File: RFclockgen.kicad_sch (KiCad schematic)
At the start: 13 parts, among them J1 Conn_01x04_Pin, J3 Conn_01x02_Pin, U3 AP2112K-3.3, U4 ESP32-C6-WROOM-1-N8

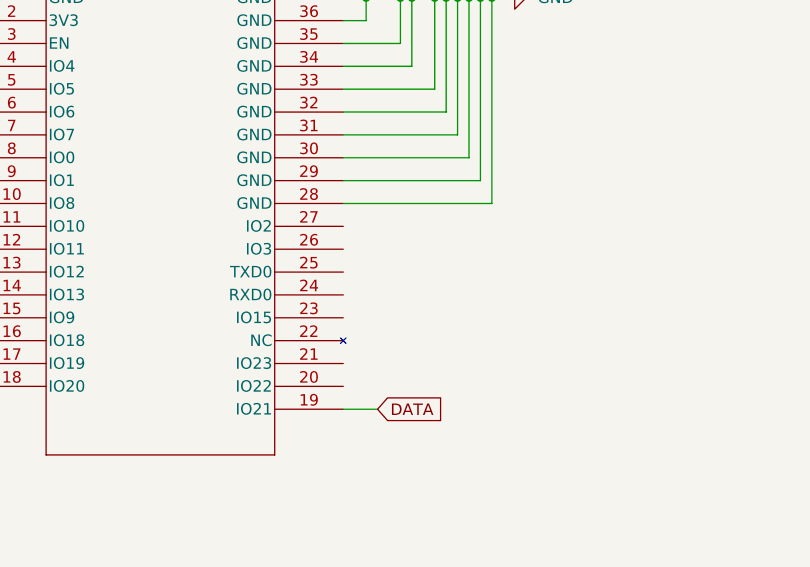
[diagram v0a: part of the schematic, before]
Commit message: Actually started on PCB layout
Started the USB C connector
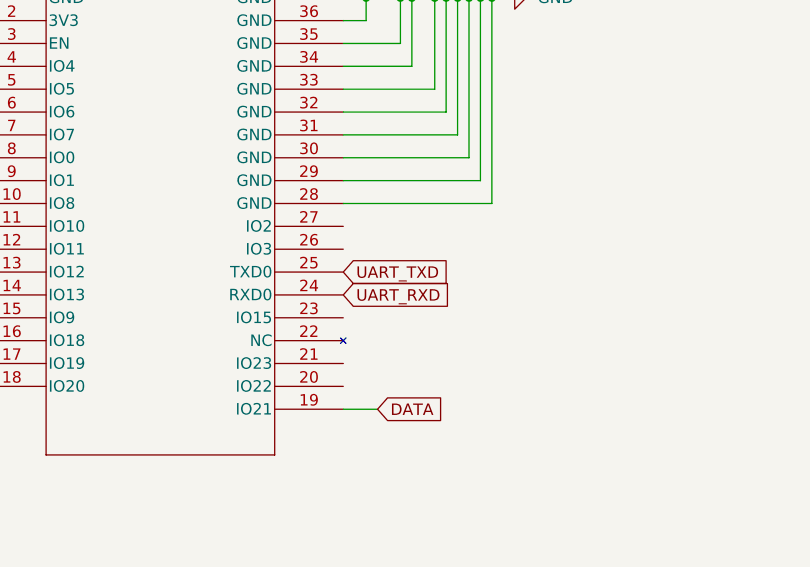
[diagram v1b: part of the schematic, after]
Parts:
- FB1, FB2: footprint (none) -> Inductor_SMD:L_1206_3216Metric_Pad1.22x1.90mm_HandSolder
- J1: footprint (none) -> Connector_PinHeader_1.00mm:PinHeader_1x04_P1.00mm_Vertical
- J3: footprint (none) -> Connector_PinHeader_1.00mm:PinHeader_1x02_P1.00mm_Vertical
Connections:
- net UART_RXD: now reaches U4.24 (RXD0)
- net UART_TXD: now reaches U4.25 (TXD0)
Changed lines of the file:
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@@
+		)
+	)
+	(global_label "UART_RXD"
+		(shape input)
+		(at 209.55 85.09 0)
+		(fields_autoplaced yes)
+		(effects
+			(font
+				(size 1.27 1.27)
+			)
+			(justify left)
+		)
+		(property "Intersheetrefs" "${INTERSHEET_REFS}"
+			(at 221.909 85.09 0)
+			(effects
+				(font
+					(size 1.27 1.27)
+				)
+				(justify left)
+				(hide yes)
+			)
 		)
 	)
@@
 		)
 	)
+	(global_label "UART_TXD"
+		(shape input)
+		(at 209.55 82.55 0)
+		(fields_autoplaced yes)
+		(effects
+			(font
+				(size 1.27 1.27)
+			)
+			(justify left)
+		)
+		(property "Intersheetrefs" "${INTERSHEET_REFS}"
+			(at 221.6066 82.55 0)
+			(effects
+				(font
+					(size 1.27 1.27)
+				)
+				(justify left)
+				(hide yes)
+			)
+		)
+	)
 	(symbol
 		(lib_id "power:GND")
@@
 			)
 		)
-		(property "Footprint" ""
+		(property "Footprint" "Connector_PinHeader_1.00mm:PinHeader_1x04_P1.00mm_Vertical"
 			(at 149.86 62.23 0)
 			(effects
@@
 			)
 		)
-		(property "Footprint" ""
+		(property "Footprint" "Inductor_SMD:L_1206_3216Metric_Pad1.22x1.90mm_HandSolder"
 			(at 148.59 144.018 90)
 			(effects
@@
 			)
 		)
-		(property "Footprint" ""
+		(property "Footprint" "Connector_PinHeader_1.00mm:PinHeader_1x02_P1.00mm_Vertical"
 			(at 149.86 87.63 0)
 			(effects
@@
 			)
 		)
-		(property "Footprint" ""
+		(property "Footprint" "Inductor_SMD:L_1206_3216Metric_Pad1.22x1.90mm_HandSolder"
 			(at 134.112 127 90)
 			(effects
